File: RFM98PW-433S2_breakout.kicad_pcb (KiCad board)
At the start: 2 copper layers, 27.4 x 48.3 mm, 14 parts, among them J1 U.FL-R-SMT-1(10), J2 Conn_01x05_Male, J3 Conn_01x03_Male, J4 Conn_01x02_Male, J5 Conn_01x02_Male, J6 Conn_01x02_Male, U1 RFM98PW-433S2

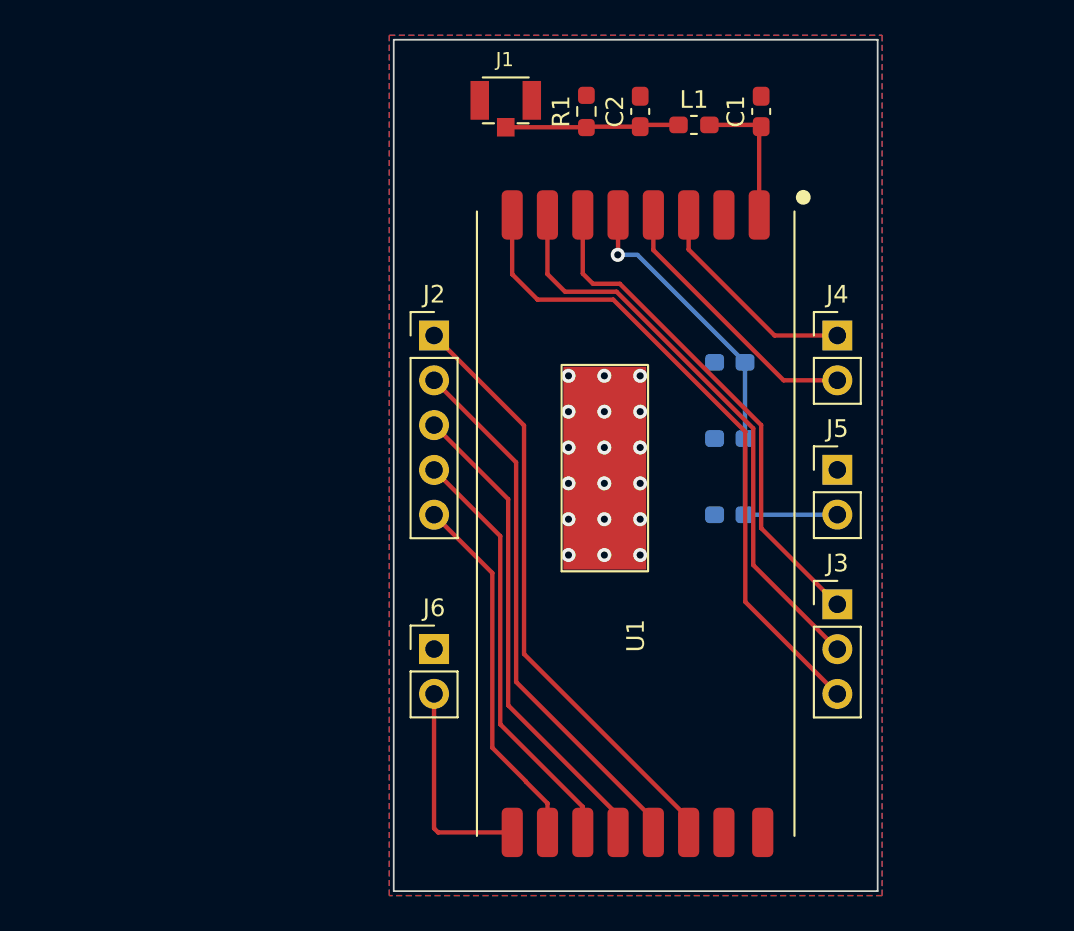
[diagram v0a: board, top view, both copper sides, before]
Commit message: first run
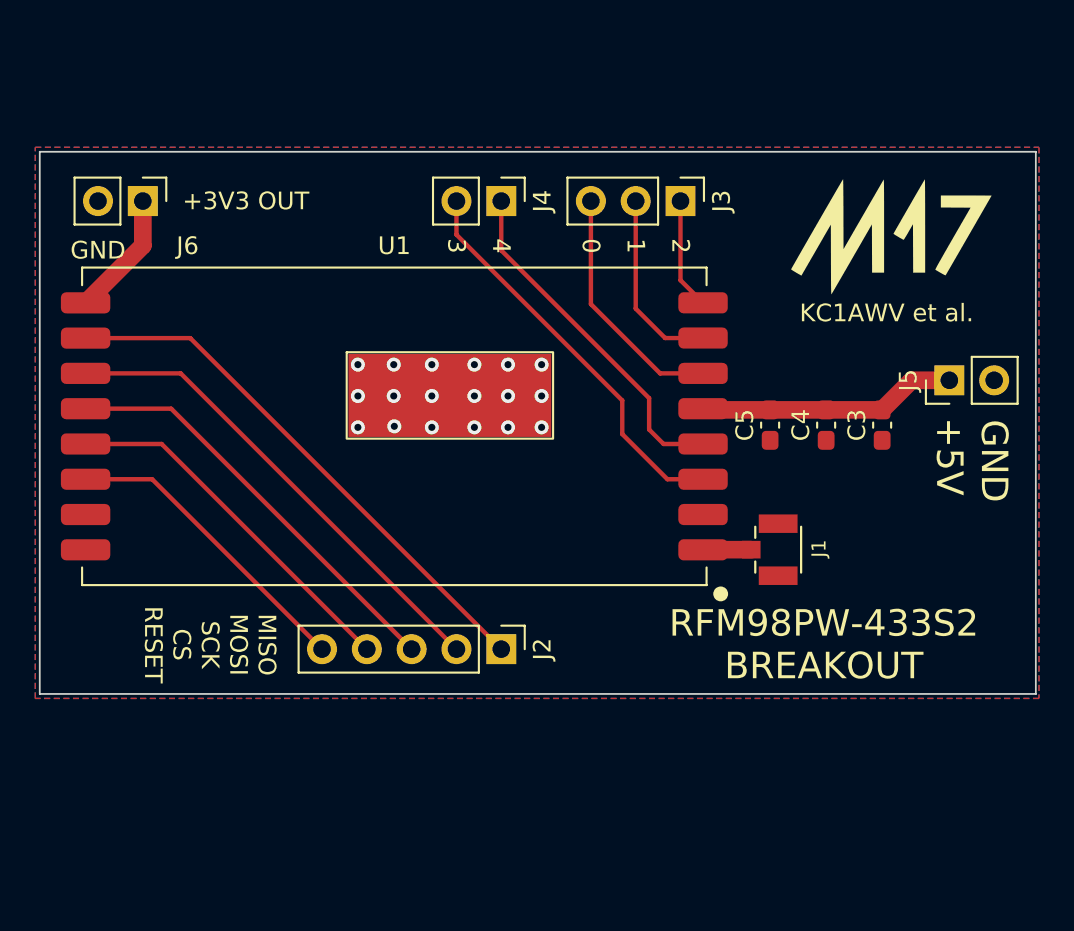
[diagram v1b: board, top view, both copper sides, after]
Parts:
- removed C1, C2: 6p, Capacitor_SMD:C_0603_1608Metric_Pad1.08x0.95mm_HandSolder
- removed L1: 18n, Inductor_SMD:L_0603_1608Metric_Pad1.05x0.95mm_HandSolder
- removed R1: 1M, Resistor_SMD:R_0603_1608Metric_Pad0.98x0.95mm_HandSolder
- added G1: LOGO, M17:M17, F.Cu at (166.9, 88.4)
- C3, C4, C5: moved to F.Cu
- moved J6 30.3 mm to (124.5, 86.4), turned to -90 degrees
- moved J1 29.8 mm to (160.5, 106.1), turned to -90 degrees
- moved J3 24.5 mm to (154.9, 86.4), turned to -90 degrees
- moved J4 20.5 mm to (144.8, 86.4), turned to -90 degrees
- moved J2 18.2 mm to (144.8, 111.8), turned to -90 degrees
- moved U1 14.8 mm to (138.7, 99.1), turned to 0 degrees
- moved C3 9.34 mm to (166.4, 99.1), turned to 90 degrees
- moved J5 8.13 mm to (170.2, 96.5), turned to 90 degrees
- moved C5 5.57 mm to (160.0, 99.1), turned to 90 degrees
- moved C4 5.51 mm to (163.2, 99.1), turned to 90 degrees
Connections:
- J1 pad 2: Net-(L1-Pad1) -> Net-(J1-Pad2)
- J2 pad 1: RFM_RESET -> RFM_MISO
- J2 pad 2: RFM_NSS -> RFM_MOSI
- J2 pad 4: RFM_MOSI -> RFM_NSS
- J2 pad 5: RFM_MISO -> RFM_RESET
- J3 pad 1: RFM_DIO0 -> RFM_DIO2
- J3 pad 3: RFM_DIO2 -> RFM_DIO0
- J4 pad 1: RFM_DIO3 -> RFM_DIO4
- J4 pad 2: RFM_DIO4 -> RFM_DIO3
- J5 pad 1: GND -> +5V
- J5 pad 2: +5V -> GND
- J6 pad 1: GND -> +3V3
- J6 pad 2: +3V3 -> GND
- U1 pad 1: Net-(C1-Pad1) -> Net-(J1-Pad2)
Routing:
- net RFM_DIO2: track 37.3 -> 6.30 mm
- net RFM_DIO1: track 33.1 -> 10.6 mm
- net RFM_RESET: track 34.1 -> 17.4 mm
- net RFM_DIO0: track 28.9 -> 13.8 mm
- net +5V: track 25.9 -> 14.7 mm, vias 1 -> 0
- net RFM_DIO3: track 12.4 -> 22.7 mm
- net RFM_MISO: track 20.7 -> 30.9 mm
- net Net-(L1-Pad1): track 10.1 -> 0.00 mm
- net RFM_NSS: track 30.8 -> 20.8 mm
- net Net-(C1-Pad1): track 7.77 -> 0.00 mm
- net +3V3: track 12.1 -> 7.11 mm
- net RFM_DIO4: track 15.5 -> 19.8 mm
- net RFM_MOSI: track 24.0 -> 27.5 mm
- net RFM_SCK: track 27.4 -> 24.1 mm
- net Net-(J1-Pad2): track 0.00 -> 2.74 mm
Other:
- board size 27.4 x 48.3 mm -> 56.5 x 30.7 mm
- board text added: "+3V3 OUT"
- board text added: "+5V"
- board text added: "0"
- board text added: "1"
- board text added: "2"
- board text added: "3"
- board text added: "4"
- board text added: "GND"
- board text added: "KC1AWV et al."
- board text added: "MISO MOSI SCK CS RESET"
- board text added: "RFM98PW-433S2 BREAKOUT"
- board text added: "write something."
